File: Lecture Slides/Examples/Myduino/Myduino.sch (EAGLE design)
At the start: 30 parts, among them J2 GENERIC-BATTERY-CONN-RECEPTAC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, SW1 PUSHBUTTON-SHIELD-GND_CK_KMR2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, U1 ATMEGA328-NO-THERMAL_32TQFP, U3 ADJUSTABLE-VOLTAGE-REGULATOR_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, Y1 16MHz

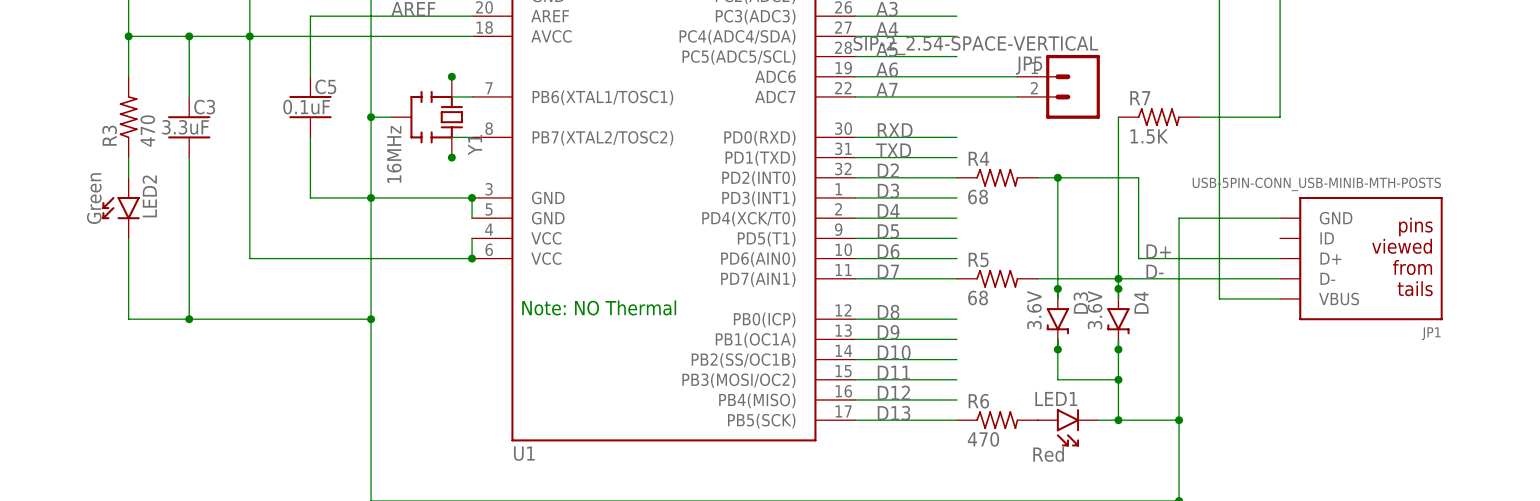
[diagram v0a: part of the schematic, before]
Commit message: new slides
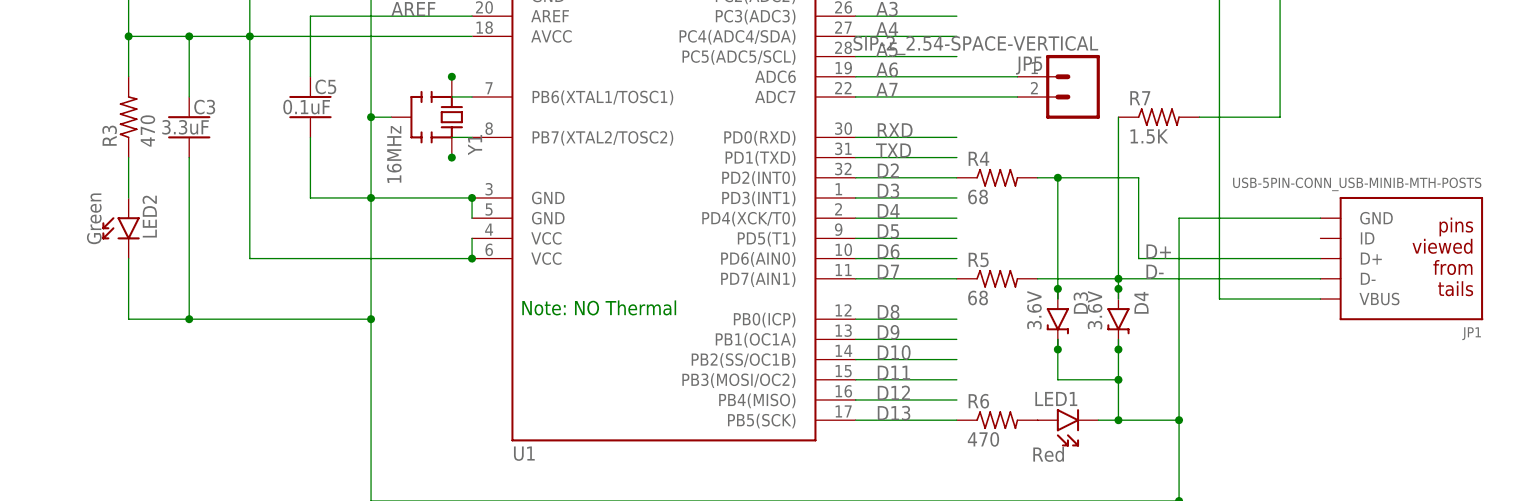
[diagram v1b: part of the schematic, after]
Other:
- moved on the sheet: JP1, LED2
